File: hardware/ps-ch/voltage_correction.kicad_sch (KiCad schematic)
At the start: 43 parts, among them Q10 MMBT3906, Q11 MMBT3904, Q12 MMBT3904, Q9 MMBT3906, U15 OPA992IDBVR, U16 OPA992IDBVR, U17 OPA992IDBVR

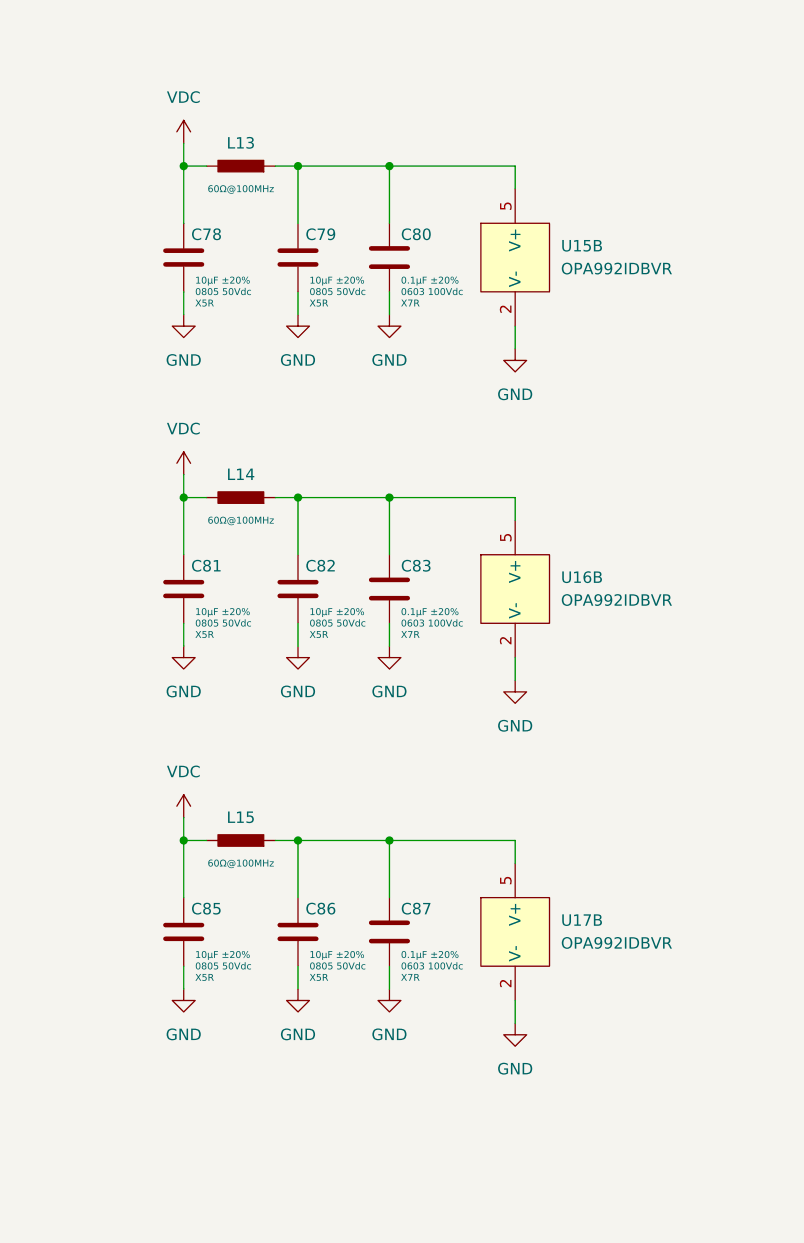
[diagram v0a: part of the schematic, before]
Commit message: started floorplanning
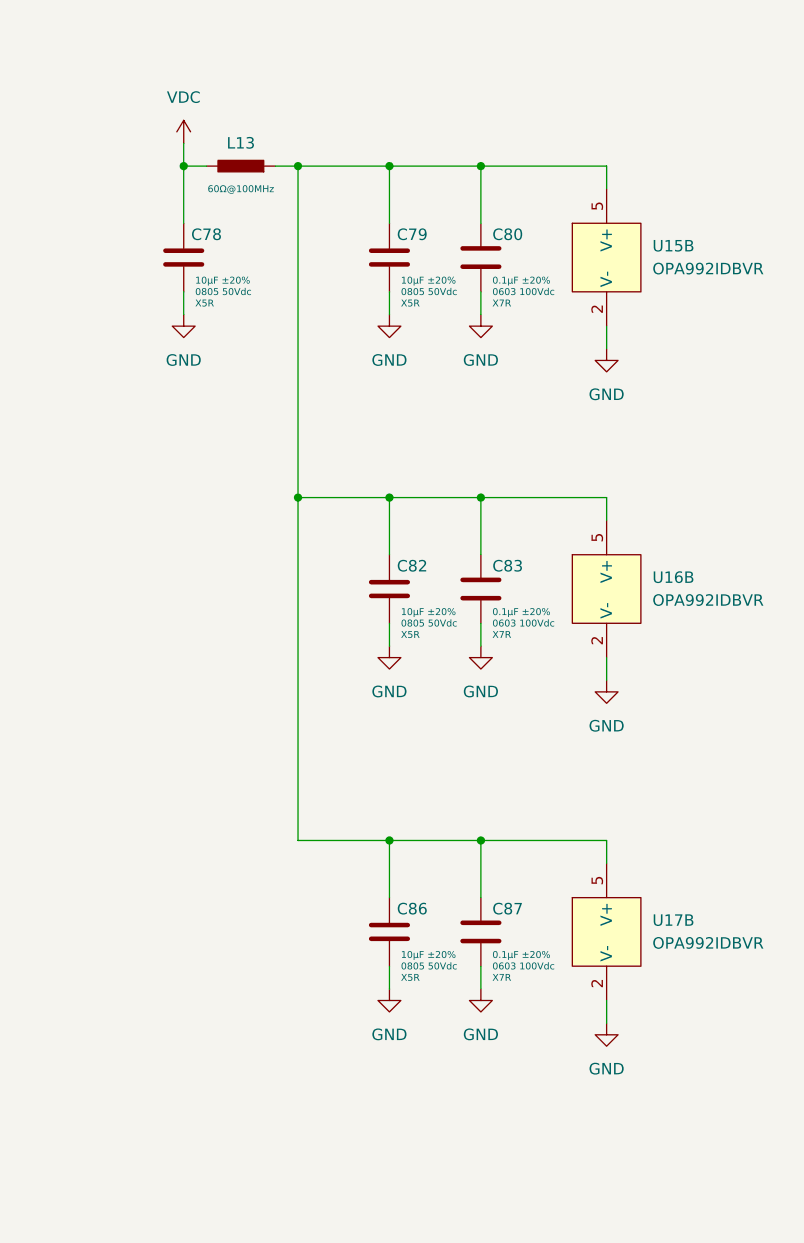
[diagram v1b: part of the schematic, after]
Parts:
- removed C81, C85: 10μF 0805 50Vdc X5R ±20%, Capacitor_SMD:C_0805_2012Metric, symbol ps-ch:10μF 0805 50Vdc X5R ±20%
- removed L14, L15: 60Ω@100MHz, Inductor_SMD:L_0603_1608Metric, symbol ps-ch:74437349015
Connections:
- net at C79.2, C80.2, L13.1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: now also C82.2, C83.2, C86.2, C87.2, U16.5 (V+), U17.5 (V+)
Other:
- moved on the sheet: C79, C80, C82, C83, C86, C87, U15B, U16B, U17B
